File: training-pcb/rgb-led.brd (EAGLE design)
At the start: 30 x 30 mm, 23 parts, among them J1 MICRO-USB, J2 AVR_SPI_PROG2PTH2, U1 ATTINY441/841SSU/SSUR, U2 PCA9533

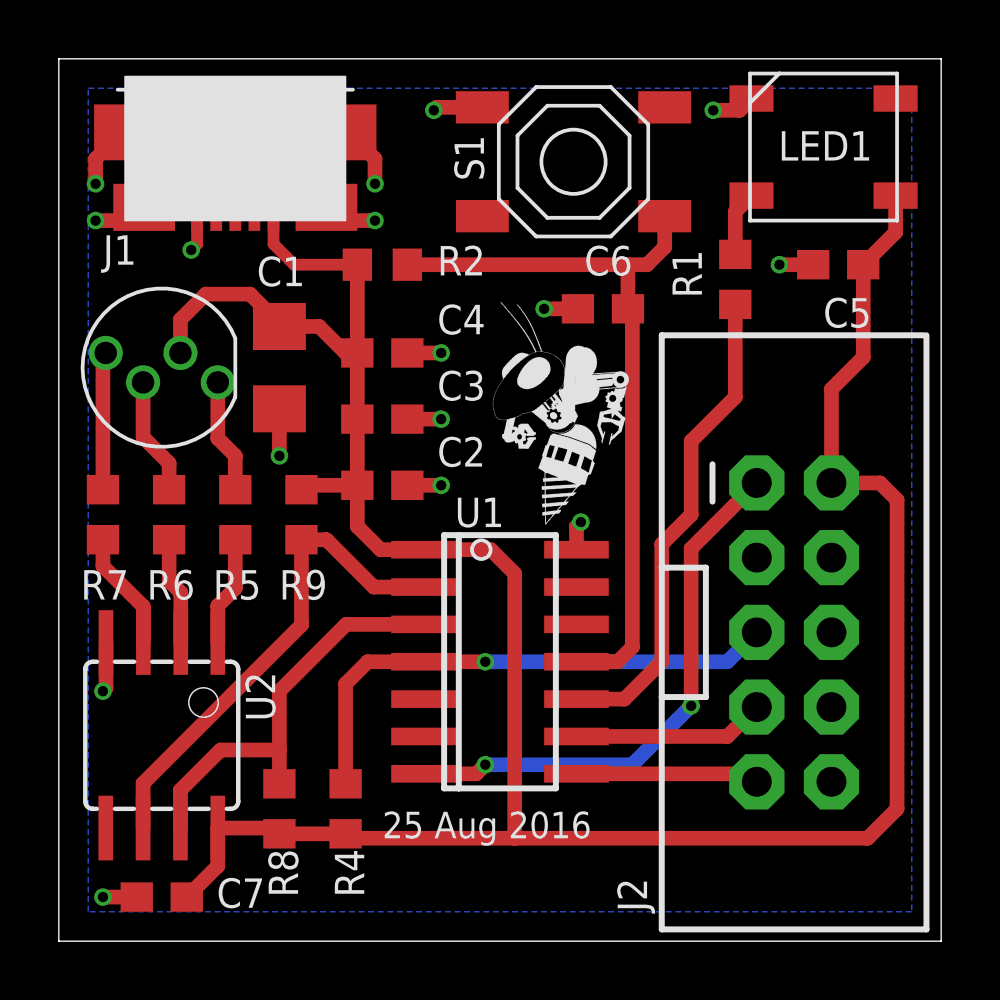
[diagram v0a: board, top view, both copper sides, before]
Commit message: updated avrdude.conf
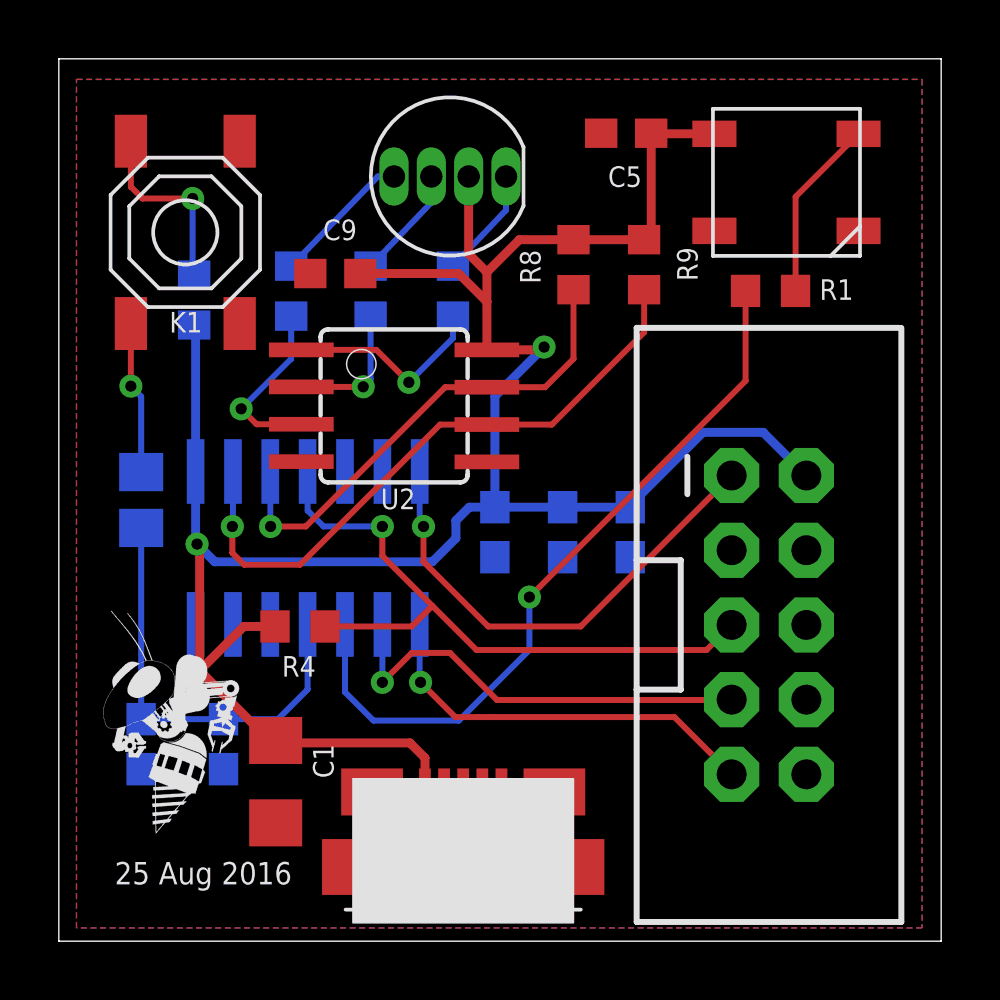
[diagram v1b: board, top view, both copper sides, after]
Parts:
- removed S1: SKQGADE010, Seeed-OPL-Button:SW4-SMD-5.2X5.2X1.5MM
- added C9: 100n, rcl:C0603
- added K1: SKQGADE010, rgb-led:SW4-SMD-5.2X5.2X1.5MM
- added R3: 39K, resistor:R0805
- C1: value 47uF -> 47u
- C2, C3, C4, C5, C6, C7: value 0.1uF -> 100n
- R2, R8, R9: value 10k -> 10K
- U2: device adam - ics:SOIC8 -> rgb-led:SOIC8
- moved J1 26.2 mm to (13.7, 2.52), turned to 0 degrees
- moved R8 21.0 mm to (17.5, 23.0), turned to 90 degrees
- moved C6 19.6 mm to (5.60, 6.70), flipped to the bottom, turned to 270 degrees
- moved U$2 16.9 mm to (3.28, 3.66)
- moved R9 14.4 mm to (19.9, 23.0)
- moved C1 14.1 mm to (7.37, 5.42)
- moved U2 13.7 mm to (11.4, 18.2), turned to 270 degrees
- moved D1 11.8 mm to (13.3, 26.0)
- moved R5 10.6 mm to (13.4, 22.1), flipped to the bottom
- moved C4 10.4 mm to (19.4, 13.9), flipped to the bottom, turned to 270 degrees
- moved R6 10.2 mm to (10.6, 22.1), flipped to the bottom
- moved R7 9.94 mm to (7.90, 22.1), flipped to the bottom
- moved C5 8.48 mm to (19.3, 27.5)
- moved U1 7.60 mm to (8.46, 13.4), flipped to the bottom, turned to 180 degrees
- moved C3 7.23 mm to (17.1, 13.9), flipped to the bottom, turned to 270 degrees
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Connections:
- net !RESET renamed /RESET
- removed net !BTN: C6.1, R2.1, S1.1, U1.11
- new net /BTN: C6.1, C7.1, R3.2, U1.11
- new net N$2: K1.2, R2.1
- new net N$3: K1.1, R3.1
- net +5V: now also C9.1; no longer C7.1
- net GND: now also C9.2, K1.3; no longer S1.3
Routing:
- net GND: track 31.4 -> 0.00 mm, vias 16 -> 0
- net !BTN: track 25.2 -> 0.00 mm
- net /BTN: track 0.00 -> 14.8 mm
- net +5V: track 88.6 -> 79.6 mm, vias 0 -> 2
- net LED_CNTRL: track 16.6 -> 25.2 mm, vias 0 -> 1
- net SCK: track 6.54 -> 14.9 mm, vias 0 -> 1
- net MISO: track 6.24 -> 13.9 mm, vias 0 -> 1
- net N$2: track 0.00 -> 6.42 mm, vias 0 -> 1
- net N$3: track 0.00 -> 5.19 mm, vias 0 -> 1
- net SCL: track 16.9 -> 21.7 mm, vias 0 -> 1
- net /RESET: track 18.1 -> 22.6 mm
- net N$1: track 2.23 -> 6.23 mm
- net N$11: track 3.74 -> 6.98 mm, vias 0 -> 1
- net SDA: track 14.2 -> 16.9 mm, vias 0 -> 1
- net N$13: track 4.07 -> 6.12 mm, vias 0 -> 1
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- added copper zone on layer 1, net GND
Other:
- board text removed: "J1"
- board text removed: "J2"
